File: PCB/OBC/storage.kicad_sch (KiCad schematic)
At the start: 2 parts, among them U1 W25Q128JVSIQ

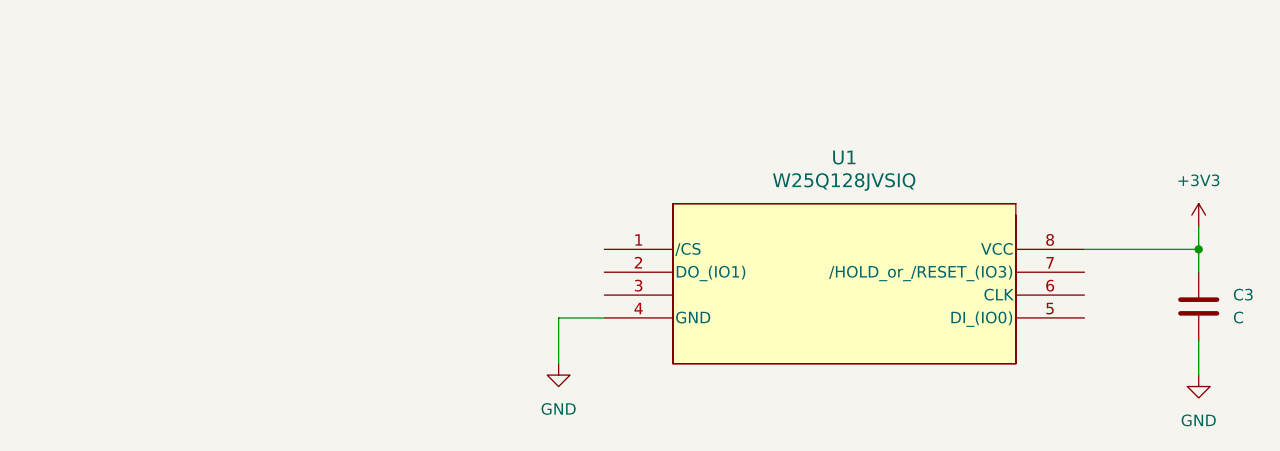
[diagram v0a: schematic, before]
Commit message: Watchdog
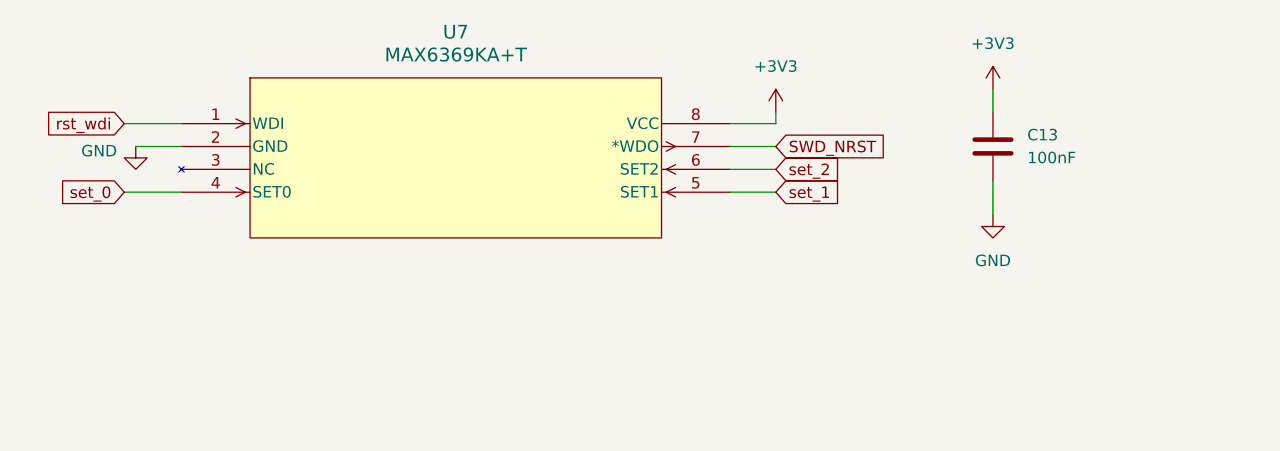
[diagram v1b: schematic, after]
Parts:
- removed C3: C, symbol Device:C
- removed U1: W25Q128JVSIQ, SOIC_128JVSIQ_WIN, symbol W25Q128JVSIQ:W25Q128JVSIQ
- added C13: 100nF, symbol Device:C
- added U7: MAX6369KA+T, 21-0078H_MXM, symbol MAX6369KA+T:MAX6369KA+T
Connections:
- net +3V3: now also C13.1, U7.8 (VCC)
- net GND: now also C13.2, U7.2 (GND)
- new net SWD_NRST: U7.7 (*WDO)
- new net rst_wdi: U7.1 (WDI)
- new net set_0: U7.4 (SET0)
- new net set_1: U7.5 (SET1)
- new net set_2: U7.6 (SET2)
